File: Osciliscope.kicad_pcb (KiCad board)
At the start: 2 copper layers, 135.1 x 85.3 mm, 31 parts, among them J1 USB_C_Receptacle_USB2.0_14P, J2 Conn_ARM_JTAG_SWD_20, U1 STM32H753VITx, X1 X322525MOB4SI

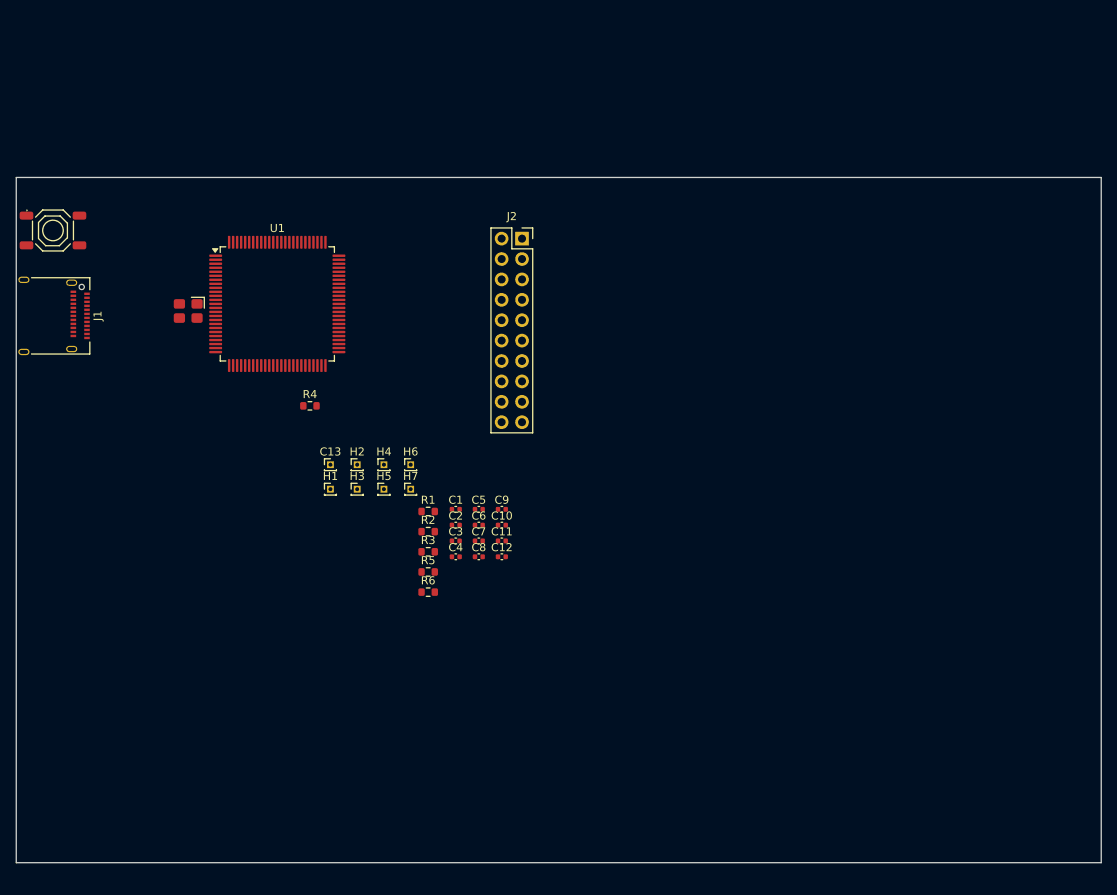
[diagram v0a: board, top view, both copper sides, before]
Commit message: Basic PCB
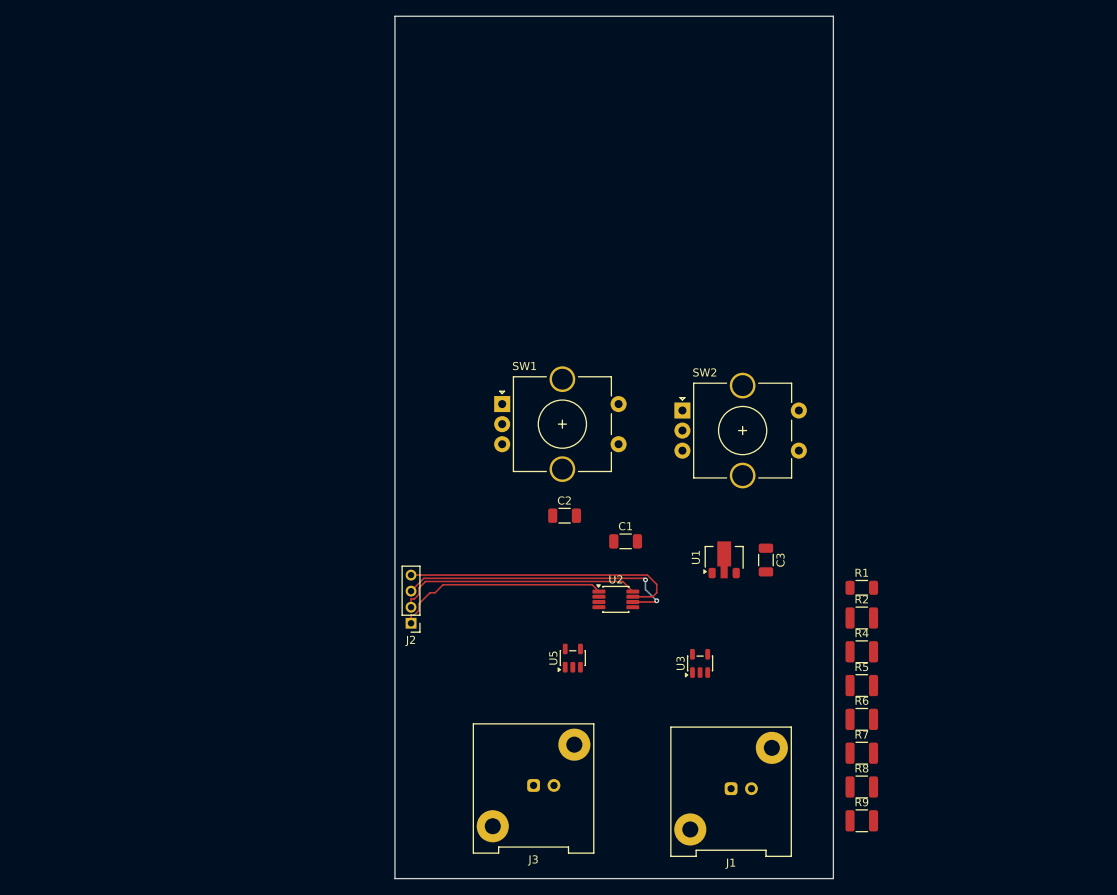
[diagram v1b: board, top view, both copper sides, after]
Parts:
- removed C10, C11, C12, C4: 100n, Capacitor_SMD:C_0402_1005Metric
- removed C13: 100n, Connector_PinHeader_1.00mm:PinHeader_1x01_P1.00mm_Vertical
- removed C5, C6: 2.2u, Capacitor_SMD:C_0402_1005Metric
- removed C7: 0.1u, Capacitor_SMD:C_0402_1005Metric
- removed C8, C9: 3.9pf, Capacitor_SMD:C_0402_1005Metric
- removed H1, H2, H3, H4, H5, H6, H7: MountingHole_Pad, Connector_PinHeader_1.00mm:PinHeader_1x01_P1.00mm_Vertical
- removed R3: 5.1k, Resistor_SMD:R_0603_1608Metric
- removed S1: Tactile Button, 160gf, PCM_JLCPCB:SW-SMD_4P-L5.1-W5.1-P3.70-LS6.5-TL-2
- removed X1: X322525MOB4SI, PCM_JLCPCB:OSC-SMD_4P-L3.2-W2.5-BL
- added J3: U.FL, Connector_Coaxial:BNC_Amphenol_031-5539_Vertical, F.Cu at (142.7, 125.0)
- added R7: 1M, Resistor_SMD:R_1210_3225Metric, F.Cu at (183.5, 121.0)
- added R8: 1M, Resistor_SMD:R_1210_3225Metric, F.Cu at (183.5, 125.2)
- added R9: 1M, Resistor_SMD:R_1210_3225Metric, F.Cu at (183.5, 129.4)
- added SW1: SW_Rotary_1x8_MP, Rotary_Encoder:RotaryEncoder_Alps_EC11E-Switch_Vertical_H20mm_CircularMountingHoles, F.Cu at (138.8, 77.5)
- added SW2: SW_Rotary_1x8_MP, Rotary_Encoder:RotaryEncoder_Alps_EC11E-Switch_Vertical_H20mm_CircularMountingHoles, F.Cu at (161.2, 78.3)
- added U2: ADC082S101, Package_SO:VSSOP-8_3x3mm_P0.65mm, F.Cu at (152.9, 101.8)
- added U3: TLV9061xDBV, Package_TO_SOT_SMD:SOT-23-5, F.Cu at (163.4, 109.8)
- added U5: TLV9061xDBV, Package_TO_SOT_SMD:SOT-23-5, F.Cu at (147.5, 109.1)
- C1, C2, C3: value 100n -> 1uF; footprint Capacitor_SMD:C_0402_1005Metric -> Capacitor_SMD:C_1206_3216Metric
- J1: value USB_C_Receptacle_USB2.0_14P -> U.FL; footprint Connector_USB:USB_C_Receptacle_Amphenol_12401610E4-2A -> Connector_Coaxial:BNC_Amphenol_031-5539_Vertical
- J2: value Conn_ARM_JTAG_SWD_20 -> Conn_01x04_Socket; footprint Connector_PinSocket_2.54mm:PinSocket_2x10_P2.54mm_Vertical -> Connector_PinHeader_2.00mm:PinHeader_1x04_P2.00mm_Vertical
- R1: value 10k -> 1M; footprint Resistor_SMD:R_0603_1608Metric -> Resistor_SMD:R_1206_3216Metric
- R2: value 5.1k -> 1M; footprint Resistor_SMD:R_0603_1608Metric -> Resistor_SMD:R_1210_3225Metric
- R4: value 1k -> 1M; footprint Resistor_SMD:R_0603_1608Metric -> Resistor_SMD:R_1210_3225Metric
- R5, R6: value 22 -> 1M; footprint Resistor_SMD:R_0603_1608Metric -> Resistor_SMD:R_1210_3225Metric
- U1: value STM32H753VITx -> MCP1700x-330xxMB; footprint Package_QFP:LQFP-100_14x14mm_P0.5mm -> Package_TO_SOT_SMD:SOT-89-3
- moved J1 103.6 mm to (167.3, 125.4), turned to 0 degrees
- moved R4 75.2 mm to (183.5, 108.3)
- moved U1 64.0 mm to (166.4, 96.6), turned to 90 degrees
- moved R6 56.3 mm to (183.5, 116.8)
- moved R5 55.8 mm to (183.5, 112.6)
- moved R2 55.1 mm to (183.5, 104.1)
- moved R1 54.8 mm to (183.5, 100.4)
- moved J2 49.9 mm to (127.4, 104.8), turned to 180 degrees
- moved C3 38.7 mm to (171.6, 96.9), turned to -90 degrees
- moved C1 21.5 mm to (154.1, 94.6)
- moved C2 13.6 mm to (146.5, 91.4)
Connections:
- C1 pad 1: VDD -> 5Vin
- C2 pad 1: VDD -> 3.3Vo
- C3 pad 1: VDD -> 3.3Vo
- J2 pad 1: unconnected-(J2-VTREF-Pad1) -> RPI_CS
- J2 pad 2: unconnected-(J2-VCC/NC-Pad2) -> RPI_SCLK
- J2 pad 3: unconnected-(J2-~{TRST}-Pad3) -> RPI_DIN
- J2 pad 4: Net-(J2-GND-Pad10) -> RPI_DOUT
- R1 pad 1: GND -> RAW_IN_1
- R1 pad 2: Net-(U1-BOOT0) -> GND
- R2 pad 1: Net-(J1-CC1) -> RAW_IN_2
- R4 pad 1: VDD -> Net-(U3-+)
- R4 pad 2: Net-(U1-VBAT) -> GND
- R5 pad 1: Net-(J1-D--PadA7) -> CHAN_1
- R5 pad 2: D- -> Net-(U3--)
- R6 pad 1: Net-(J1-D+-PadA6) -> RAW_IN_1
- R6 pad 2: D+ -> Net-(U3--)
- U1 pad 1: unconnected-(U1-PE2-Pad1) -> GND
- U1 pad 2: unconnected-(U1-PE3-Pad2) -> 5Vin
- U1 pad 3: unconnected-(U1-PE4-Pad3) -> 3.3Vo
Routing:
- net RPI_DIN: track 0.00 -> 36.2 mm, vias 0 -> 2
- net RPI_DOUT: track 0.00 -> 35.3 mm
- net RPI_SCLK: track 0.00 -> 30.5 mm
- net RPI_CS: track 0.00 -> 26.8 mm
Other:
- board size 135.1 x 85.3 mm -> 54.6 x 107.4 mm
